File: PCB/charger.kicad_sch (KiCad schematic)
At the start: 17 parts, among them U2 BQ24072RGT

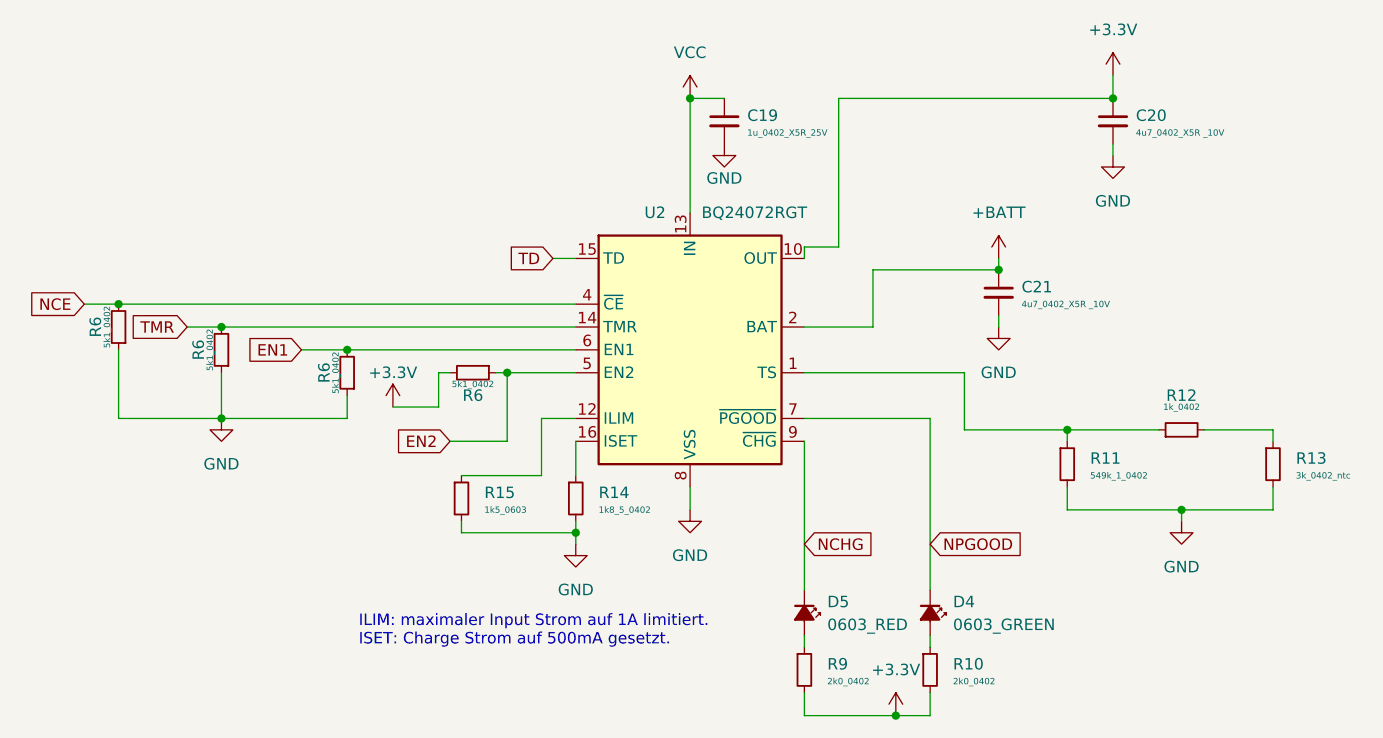
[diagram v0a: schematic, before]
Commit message: Layout weiter gemacht.
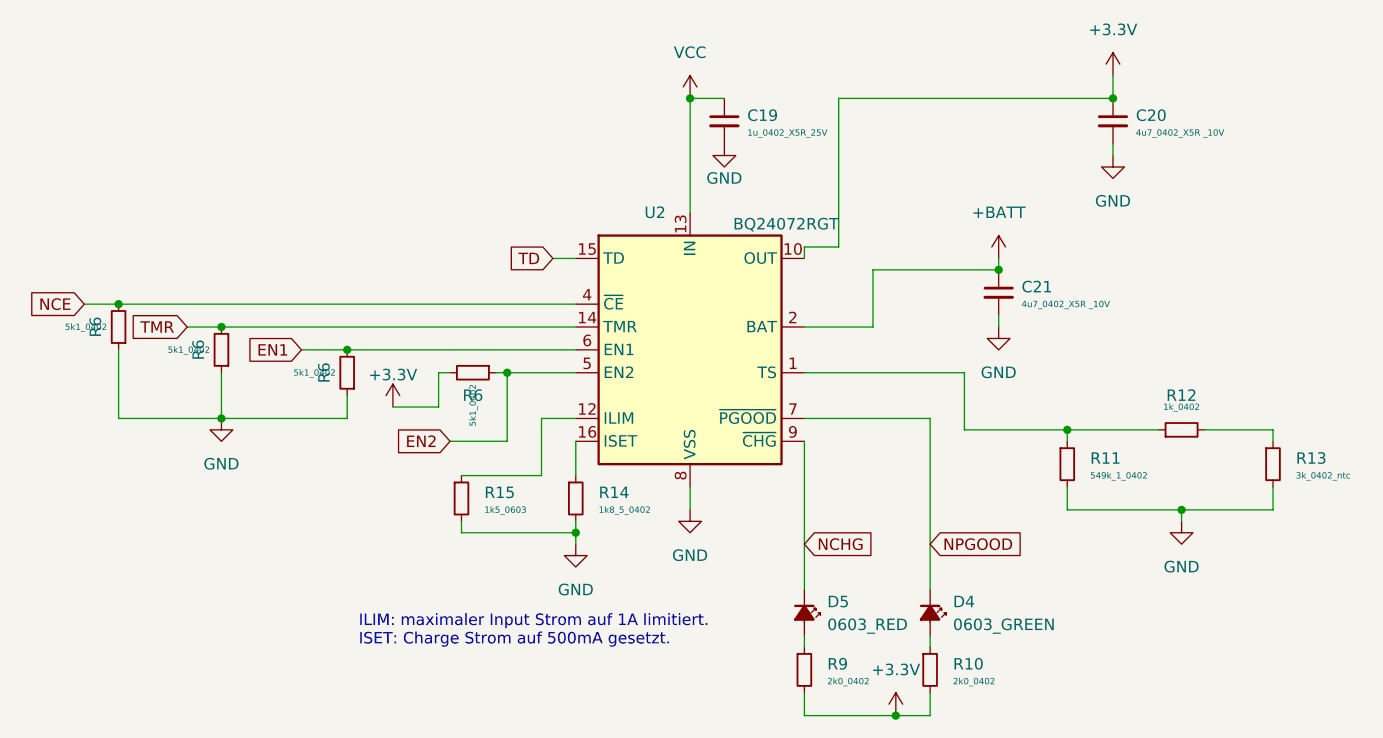
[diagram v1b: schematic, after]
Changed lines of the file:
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@@
+    )
+  )
+  (netclass_flag "" (length 2.54) (shape round) (at 162.56 72.39 0) (fields_autoplaced)
+    (effects (font (size 1.27 1.27)) (justify left bottom))
+    (property "Netclass" "BAT" (at 163.2585 69.85 0)
+      (effects (font (size 1.27 1.27) italic) (justify left))
+    )
+  )
+  (netclass_flag "" (length 2.54) (shape round) (at 135.89 59.69 90) (fields_autoplaced)
+    (effects (font (size 1.27 1.27)) (justify left bottom))
+    (property "Netclass" "Power" (at 133.35 58.9915 90)
+      (effects (font (size 1.27 1.27) italic) (justify left))
+    )
+  )
+  (netclass_flag "" (length 2.54) (shape round) (at 163.83 53.34 0) (fields_autoplaced)
+    (effects (font (size 1.27 1.27)) (justify left bottom))
+    (property "Netclass" "3V3" (at 164.5285 50.8 0)
+      (effects (font (size 1.27 1.27) italic) (justify left))
     )
   )
@@
       (effects (font (size 1.27 1.27)) hide)
     )
-    (property "Value" "+3.3V" (at 102.87 83.82 0)
+    (property "Value" "+3.3V" (at 102.87 84.074 0)
       (effects (font (size 1.27 1.27)))
     )
@@
       (effects (font (size 1.27 1.27)))
     )
-    (property "Value" "5k1_0402" (at 82.55 81.28 90)
-      (effects (font (size 0.7 0.7)))
+    (property "Value" "5k1_0402" (at 82.55 81.28 0)
+      (effects (font (size 0.7 0.7)) (justify left))
     )
     (property "Footprint" "Resistor_SMD:R_0402_1005Metric" (at 100.33 69.85 0)
@@
       (effects (font (size 1.27 1.27)))
     )
-    (property "Value" "5k1_0402" (at 111.76 85.09 90)
-      (effects (font (size 0.7 0.7)))
+    (property "Value" "5k1_0402" (at 111.76 85.09 0)
+      (effects (font (size 0.7 0.7)) (justify left))
     )
     (property "Footprint" "Resistor_SMD:R_0402_1005Metric" (at 100.33 67.31 0)
@@
       (effects (font (size 1.27 1.27)))
     )
-    (property "Value" "5k1_0402" (at 71.12 78.74 90)
-      (effects (font (size 0.7 0.7)))
+    (property "Value" "5k1_0402" (at 71.12 78.74 0)
+      (effects (font (size 0.7 0.7)) (justify left))
     )
     (property "Footprint" "Resistor_SMD:R_0402_1005Metric" (at 88.9 67.31 0)
@@
       (effects (font (size 1.27 1.27)))
     )
-    (property "Value" "5k1_0402" (at 96.52 83.82 90)
-      (effects (font (size 0.7 0.7)))
+    (property "Value" "5k1_0402" (at 96.52 83.82 0)
+      (effects (font (size 0.7 0.7)) (justify left))
     )
     (property "Footprint" "Resistor_SMD:R_0402_1005Metric" (at 114.3 72.39 0)
@@
       (effects (font (size 1.27 1.27)) (justify left))
     )
-    (property "Value" "BQ24072RGT" (at 137.16 66.04 0)
-      (effects (font (size 1.27 1.27)) (justify left))
+    (property "Value" "BQ24072RGT" (at 152.4 67.31 0)
+      (effects (font (size 1.27 1.27)) (justify right))
     )
     (property "Footprint" "Package_DFN_QFN:VQFN-16-1EP_3x3mm_P0.5mm_EP1.6x1.6mm" (at 143.51 95.25 0)

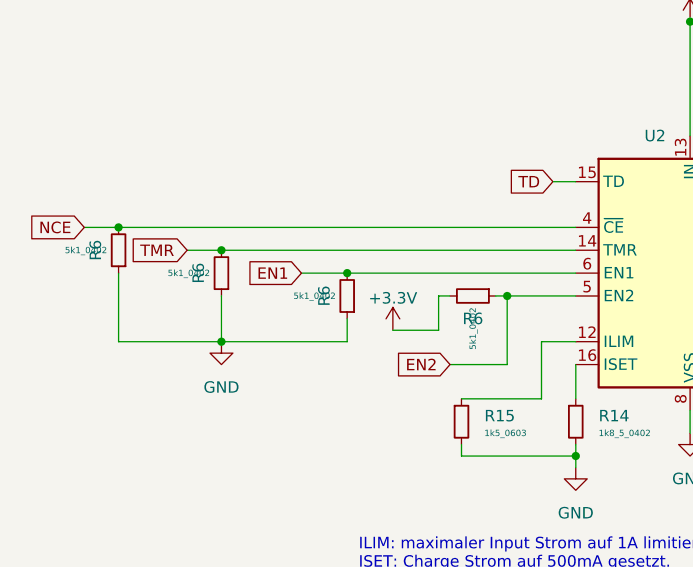
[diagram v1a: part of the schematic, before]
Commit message: update
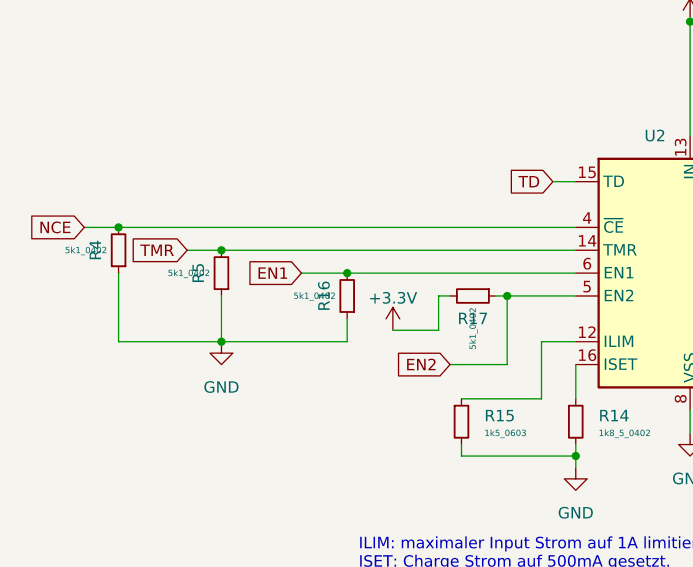
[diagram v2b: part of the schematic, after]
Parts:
- U2: LCSC (none) -> C140288
- renumbered R6 to R16, R6 to R17, R6 to R4, R6 to R5
